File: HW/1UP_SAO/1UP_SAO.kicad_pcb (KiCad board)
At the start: 2 copper layers, 48 x 48 mm, 16 parts, among them X1 Badgelife_sao_connector_v169b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

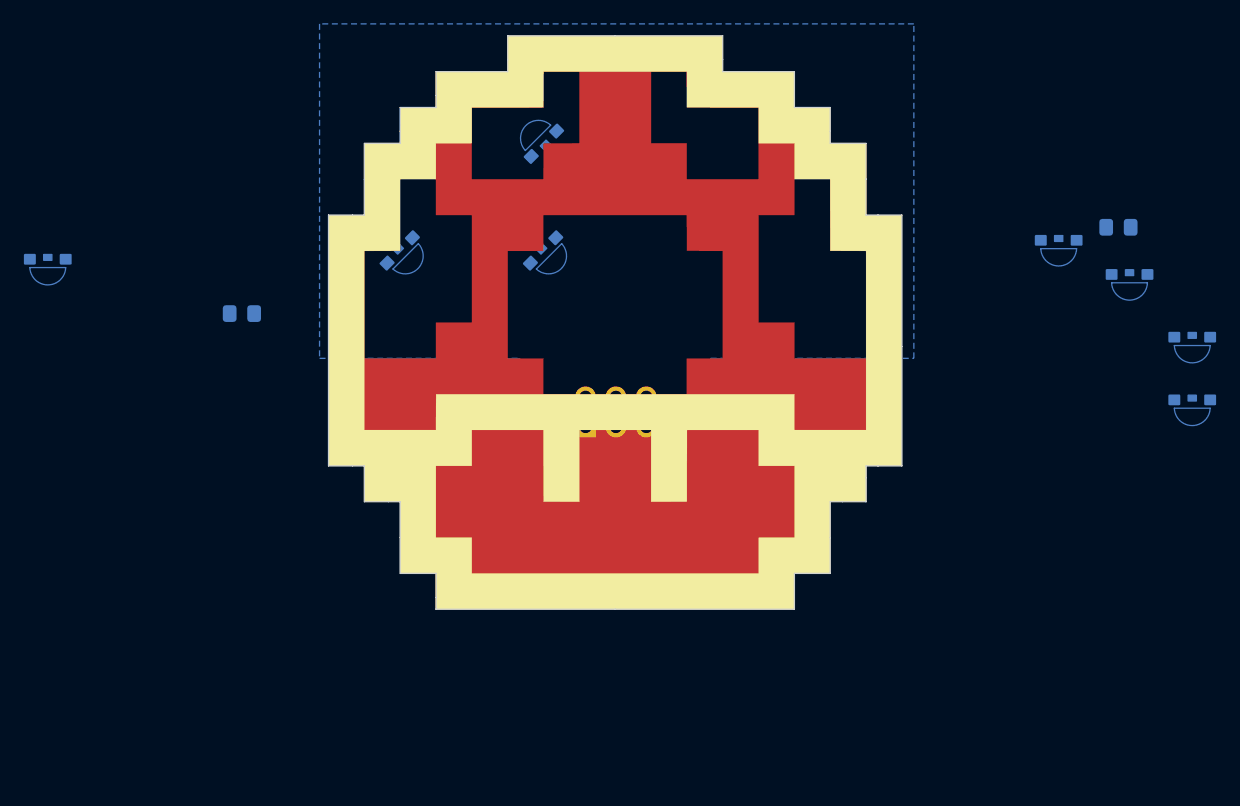
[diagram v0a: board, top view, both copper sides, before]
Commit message: moving stuff around
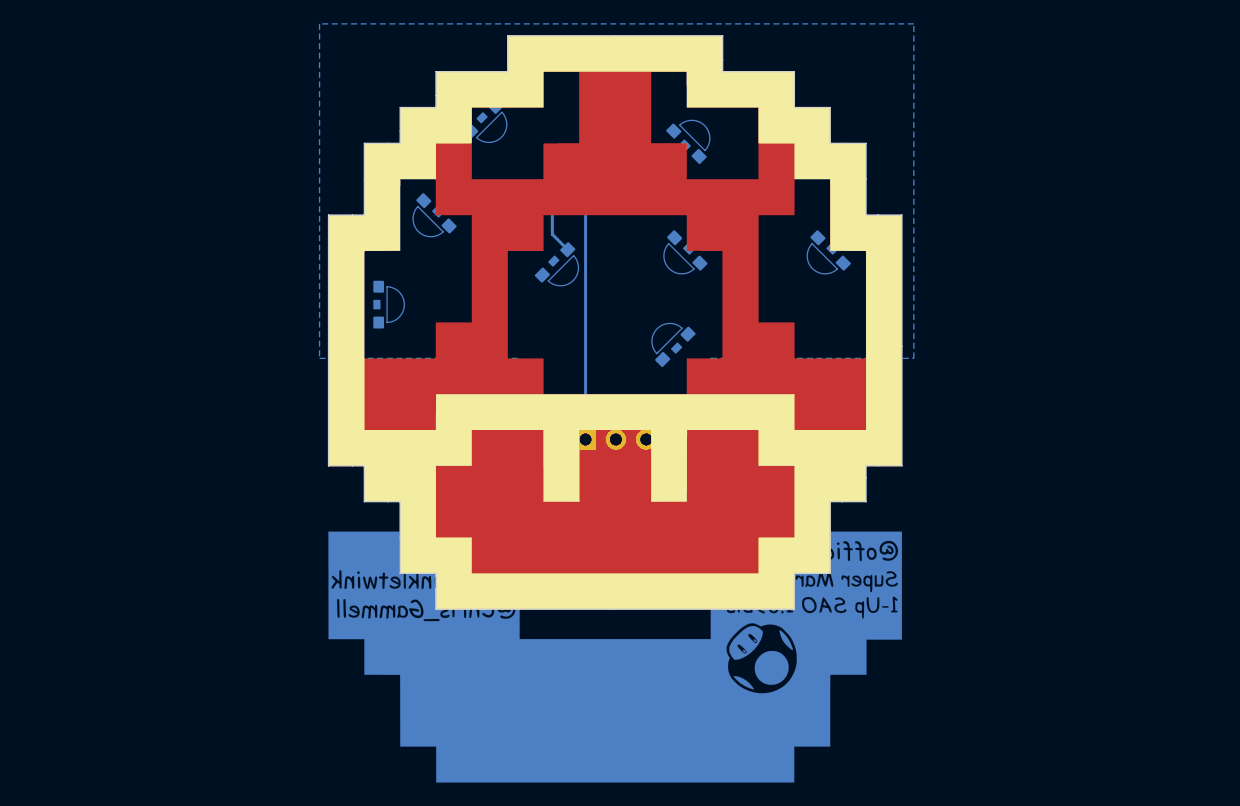
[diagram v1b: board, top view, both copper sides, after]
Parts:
- moved D5 47.5 mm to (106.0, 85.0), turned to 135 degrees
- moved De 43.3 mm to (105.0, 102.0), turned to 225 degrees
- moved R2 40.0 mm to (102.2, 89.0), turned to 90 degrees
- moved D7 37.1 mm to (106.0, 94.0), turned to 315 degrees
- moved R1 30.5 mm to (97.5, 89.0), turned to 90 degrees
- moved D4 28.0 mm to (80.2, 98.5), turned to 90 degrees
- moved D6 19.1 mm to (118.0, 94.0), turned to 315 degrees
- moved G*** 14.5 mm to (100.0, 114.5)
- moved D1 5.39 mm to (89.0, 83.0), turned to 45 degrees
- moved D3 4.32 mm to (85.0, 90.9), turned to 315 degrees
- moved D2 1.41 mm to (95.0, 95.0)
- moved X1 1.04 mm to (100.0, 108.5)
- renumbered D8 to De
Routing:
- net VCC: track 0.00 -> 22.0 mm
- net Net-(D1-Pad2): track 0.00 -> 9.03 mm
